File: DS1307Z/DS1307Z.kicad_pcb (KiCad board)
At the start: 2 copper layers, 22.9 x 20.1 mm, 14 parts, among them J1 Conn_01x06, Y1 Crystal

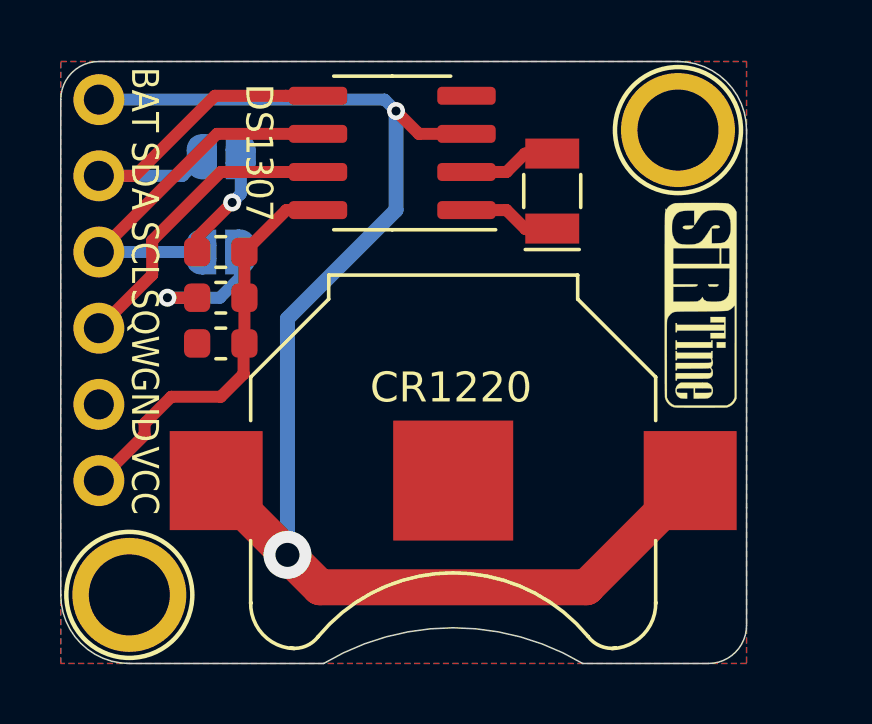
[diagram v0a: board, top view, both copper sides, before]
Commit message: DS1307ZN+ Board form factor update
Unified with DS3231
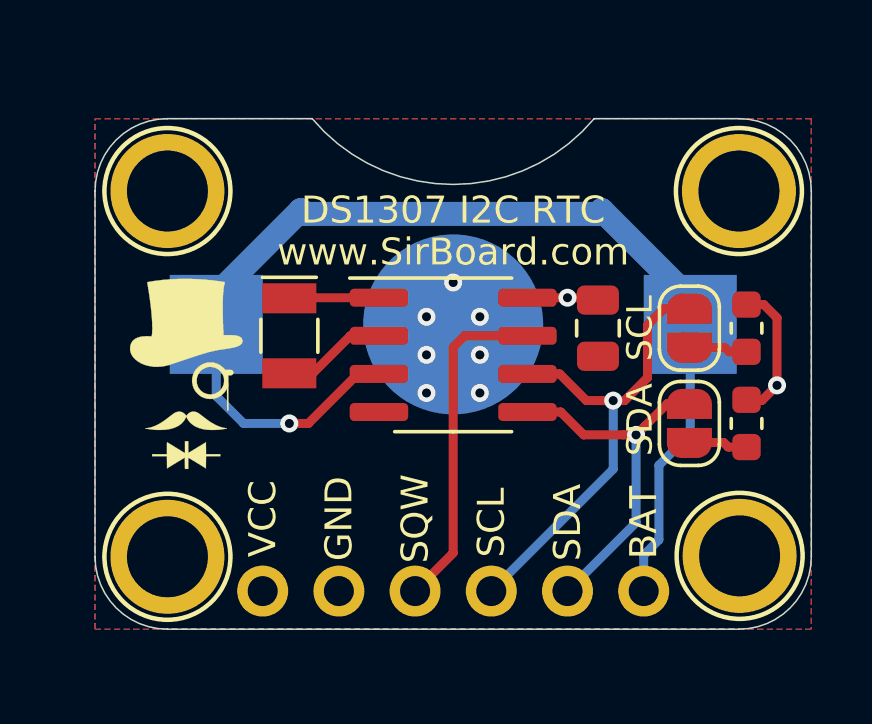
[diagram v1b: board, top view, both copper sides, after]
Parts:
- removed the G*** at (71.8, 39.0)
- removed the G*** at (64.5, 39.0)
- removed REF** (x2): MountingHole_M2.5_SirBoard, SirBoardLibrary:MountingHole_M2.5_SirBoard
- added G***: LOGO, logo:logo63x89, F.Cu at (60.6, 37.6)
- added H1: MountingHole, SirBoardLibrary:MountingHole_M2.5_SirBoard, F.Cu at (59.9, 31.5)
- added H2: MountingHole, SirBoardLibrary:MountingHole_M2.5_SirBoard, F.Cu at (59.9, 43.7)
- added H3: MountingHole, SirBoardLibrary:MountingHole_M2.5_SirBoard, F.Cu at (79.0, 31.5)
- added H4: MountingHole, SirBoardLibrary:MountingHole_M2.5_SirBoard, F.Cu at (79.0, 43.7)
- C1: footprint Capacitor_SMD:C_0603_1608Metric -> Capacitor_SMD:C_0805_2012Metric
- CR1220, G***: moved to B.Cu
- SCL, SDA: moved to F.Cu
- U1: renamed from DS1307; value DS1307Z+ -> DS1307ZN+
- Y1: value Crystal -> SMD31327681252090
- moved J1 24.5 mm to (75.8, 44.8), turned to 90 degrees
- moved R1 18.4 mm to (79.2, 39.2), turned to 90 degrees
- moved SDA 18.0 mm to (77.3, 39.2), turned to 270 degrees
- moved R2 17.6 mm to (79.2, 36.1), turned to 90 degrees
- moved SCL 15.8 mm to (77.3, 36.1), turned to 270 degrees
- moved C1 12.6 mm to (74.3, 36.1), turned to 270 degrees
- moved Y1 10.0 mm to (64.0, 36.3), turned to 270 degrees
- moved G*** 9.83 mm to (69.5, 40.6), turned to 180 degrees
- moved U1 7.03 mm to (69.5, 37.0), turned to 0 degrees
- moved CR1220 5.21 mm to (69.5, 35.9)
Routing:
- net VBAT: track 47.9 -> 38.6 mm, vias 2 -> 1
- net VCC: track 13.6 -> 7.20 mm, vias 0 -> 2
- net SCL: track 12.3 -> 16.1 mm, vias 0 -> 1
- net Net-(A2-Pad2): track 4.55 -> 1.96 mm, vias 1 -> 0
- net Net-(A1-Pad2): track 3.78 -> 1.97 mm, vias 1 -> 0
- net SQW: track 10.1 -> 11.3 mm
- net SDA: track 12.1 -> 12.3 mm, vias 0 -> 1
- net GND: vias 0 -> 7
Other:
- board size 22.9 x 20.1 mm -> 23.9 x 17 mm
- board text added: "DS1307 I2C RTC"
- board text removed: "DS1307 Based RTC"
- board text removed: "Pull-Up Delete"
